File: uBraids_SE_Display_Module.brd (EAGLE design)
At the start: 40 x 25 mm, 40 parts, among them Q1 NPN-SOT23-BEC, Q2 NPN-SOT23-BEC, Q3 NPN-SOT23-BEC, Q4 NPN-SOT23-BEC, U1 SN74HC595-TSSOP-16, U2 SN74HC595-TSSOP-16

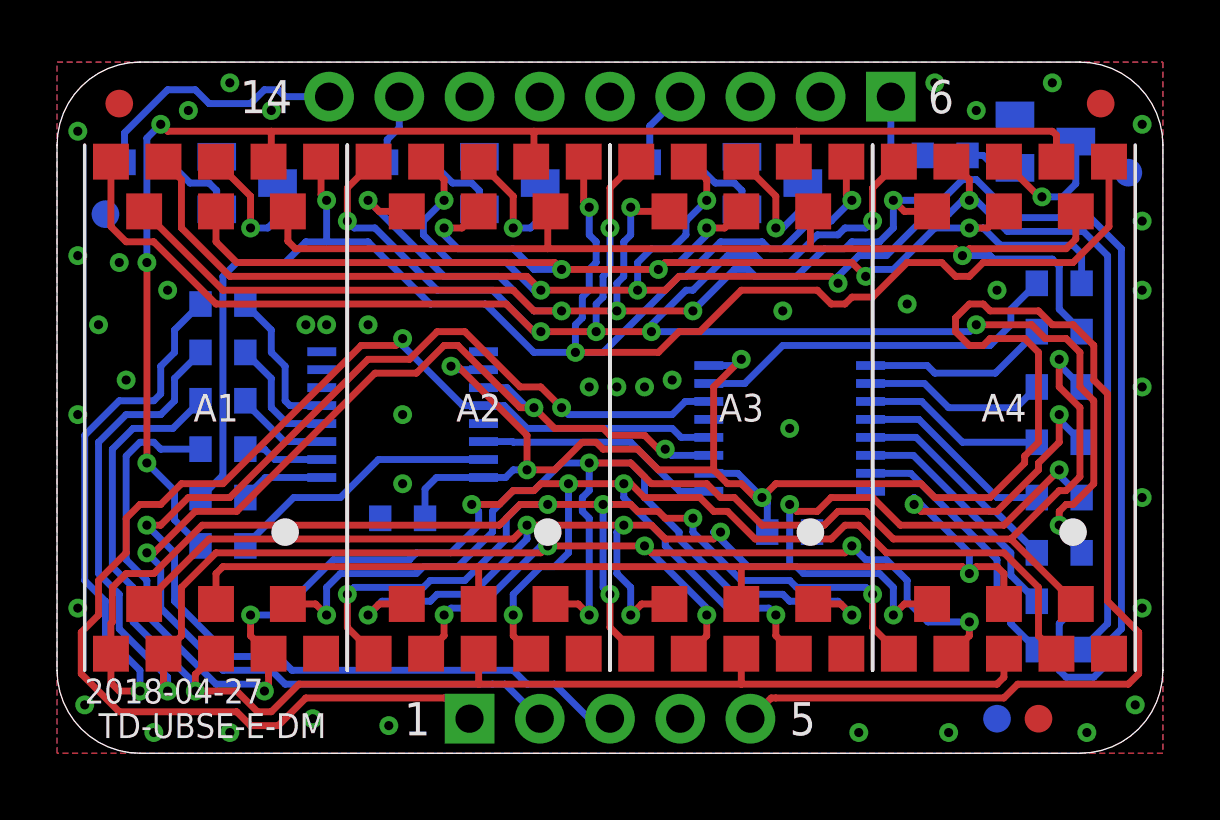
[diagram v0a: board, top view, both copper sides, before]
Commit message: Revision F
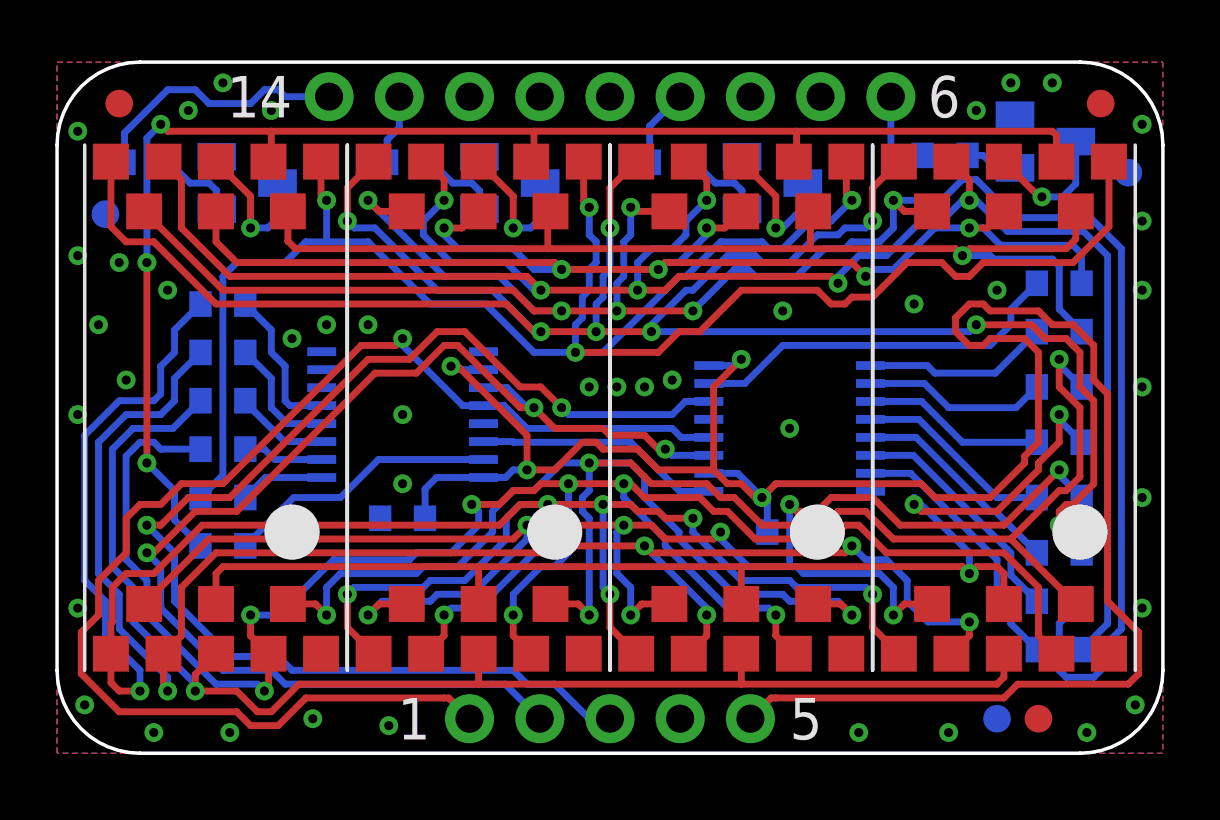
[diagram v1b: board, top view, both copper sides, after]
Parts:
- removed U$7: (no value), uBraids_SE_Library:MARKING-CC-LOGO
- removed U$8: (no value), uBraids_SE_Library:MARKING-OSH-LOGO-5MM
- A1, A2, A3, A4: device uBraids_SE_Library:14-SEGMENT-0.4"-SMD -> uBraids_SE_Library:14-SEGMENT
- H1: value HEADER-1X05-PTH-2.54-MALE -> HEADER-1X5-PTH; device uBraids_SE_Library:HEADER-1X05-PTH-2.54-MALE -> uBraids_SE_Library:PTH-0.1-1X5
- H2: value HEADER-1X09-PTH-2.54-MALE -> HEADER-1X9-PTH; device uBraids_SE_Library:HEADER-1X09-PTH-2.54-MALE -> uBraids_SE_Library:PTH-0.1-1X9
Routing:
- net N: track 64.8 -> 63.5 mm
- net L: track 71.3 -> 70.5 mm
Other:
- board text added: "C1"
- board text added: "C2"
- board text added: "C3"
- board text added: "C4"
- board text added: "TD-UBSE-F-DM 2020-02-07 tall-dog.com"
- board text removed: "2018-04-27"
- board text removed: "DC1"
- board text removed: "DC2"
- board text removed: "DC3"
- board text removed: "DC4"
- board text removed: "H1"
- board text removed: "H2"
- board text removed: "TD-UBSE-E-DM"
- board text removed: "TD-UBSE-E-DM 2018-04-27 tall-dog.com"
